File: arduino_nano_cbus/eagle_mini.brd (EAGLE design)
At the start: 71.4 x 55.9 mm, 32 parts, among them J1 1X2-3.5MM, J2 1X2-3.5MM, M1 ARDUINO-PRO-MINI-5.0V

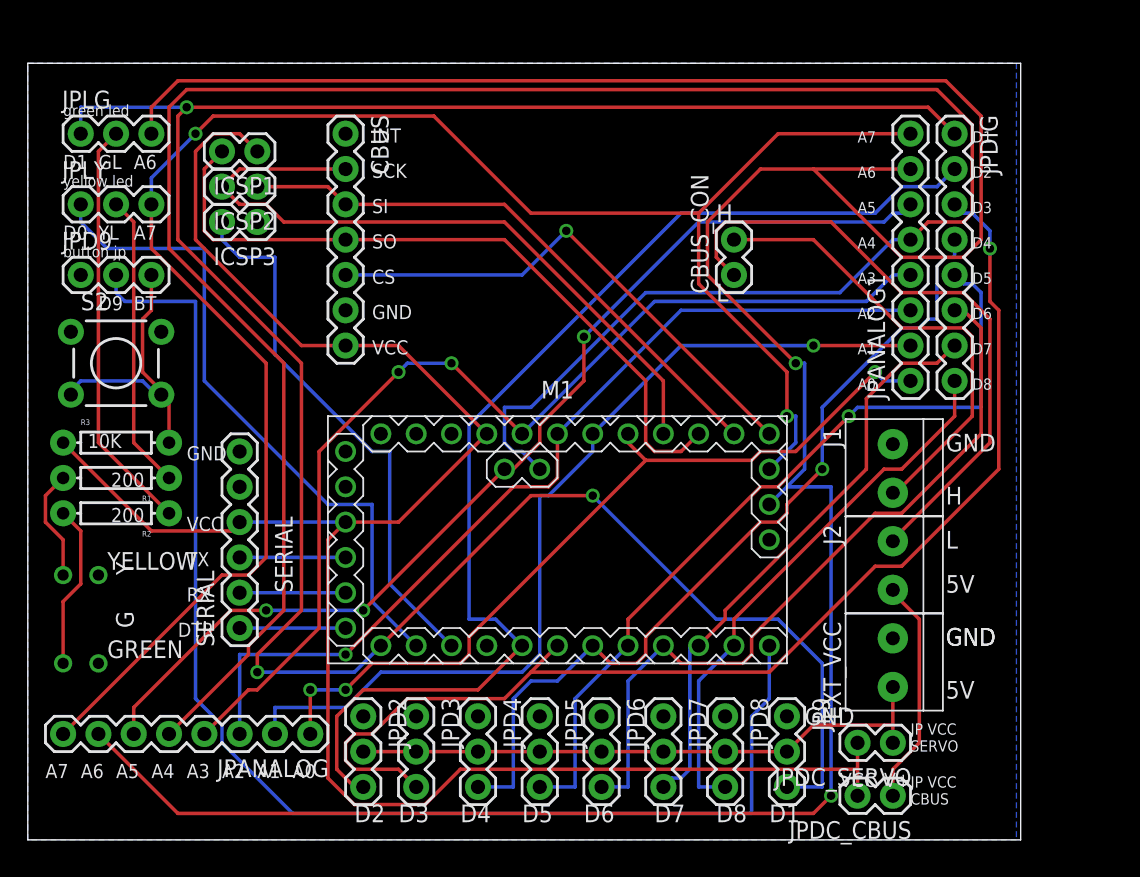
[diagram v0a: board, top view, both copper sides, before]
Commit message: some improvement on the boards.
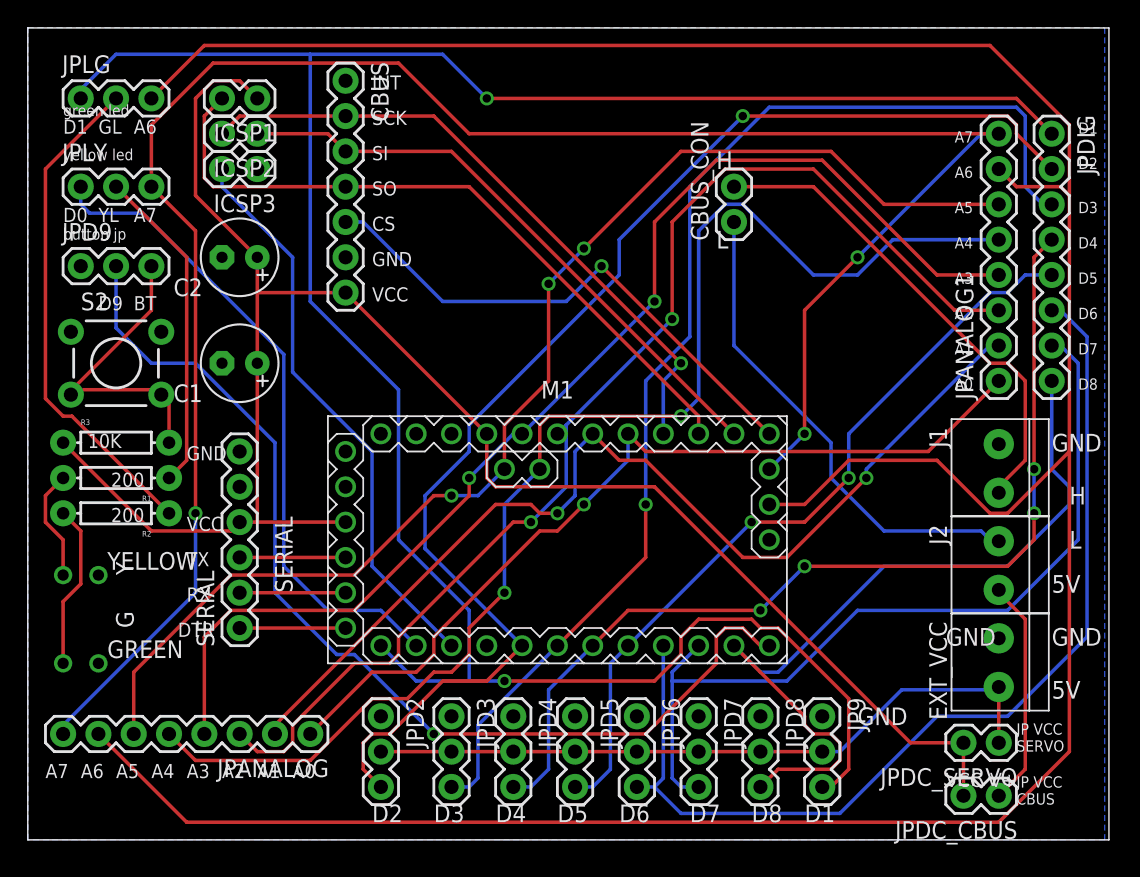
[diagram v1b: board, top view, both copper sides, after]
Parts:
- added C1, C2: 100uF, adafruit:E2,5-6
- moved EXT_VCC 7.62 mm to (69.8, 12.7)
- moved J1 7.62 mm to (69.8, 26.7)
- moved J2 7.62 mm to (69.8, 19.7)
- moved JPDC_CBUS 7.62 mm to (69.8, 3.17)
- moved JPDC_SERVO 7.62 mm to (69.8, 6.99)
- moved JPDIG 6.98 mm to (73.7, 50.8)
- moved JPANALOG1 6.35 mm to (69.8, 33.0)
- moved CBUS 3.81 mm to (22.9, 54.6)
- moved CBUS_CON 3.81 mm to (50.8, 44.5)
- moved ICSP1 3.81 mm to (16.5, 53.3)
- moved ICSP2 3.81 mm to (16.5, 50.8)
- moved ICSP3 3.81 mm to (16.5, 48.3)
- moved JPLG 2.54 mm to (3.81, 53.3)
- moved JP9 2.54 mm to (57.1, 8.89)
- moved JPD3 2.54 mm to (30.5, 8.89)
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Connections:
- net GND: now also C1.-, C2.-
- net VCC: now also C1.+, C2.+
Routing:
- net A4: track 162.9 -> 94.0 mm, vias 0 -> 2
- net A2: track 66.1 -> 85.8 mm, vias 1 -> 2
- net D6: track 54.1 -> 73.8 mm
- net D8: track 39.5 -> 58.0 mm
- net D7: track 42.7 -> 61.0 mm
- net D9: track 92.6 -> 74.7 mm, vias 0 -> 1
- net A5: track 75.4 -> 89.7 mm
- net A6: track 209.4 -> 221.8 mm, vias 2 -> 0
- net A7: track 134.8 -> 145.7 mm, vias 2 -> 3
- net D2: track 82.8 -> 92.7 mm, vias 0 -> 1
- net A3: track 76.1 -> 85.8 mm
- net L: track 45.4 -> 36.0 mm
- net A1: track 65.8 -> 74.1 mm, vias 1 -> 2
- net D4: track 62.1 -> 70.3 mm, vias 1 -> 4
- net V+: track 42.9 -> 50.5 mm
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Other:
- board size 71.4 x 55.9 mm -> 77.8 x 58.4 mm
